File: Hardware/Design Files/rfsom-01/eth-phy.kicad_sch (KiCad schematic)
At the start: 45 parts, among them U6 KSZ9131RNXI-TR, Y1 ECS-2033-500-BN

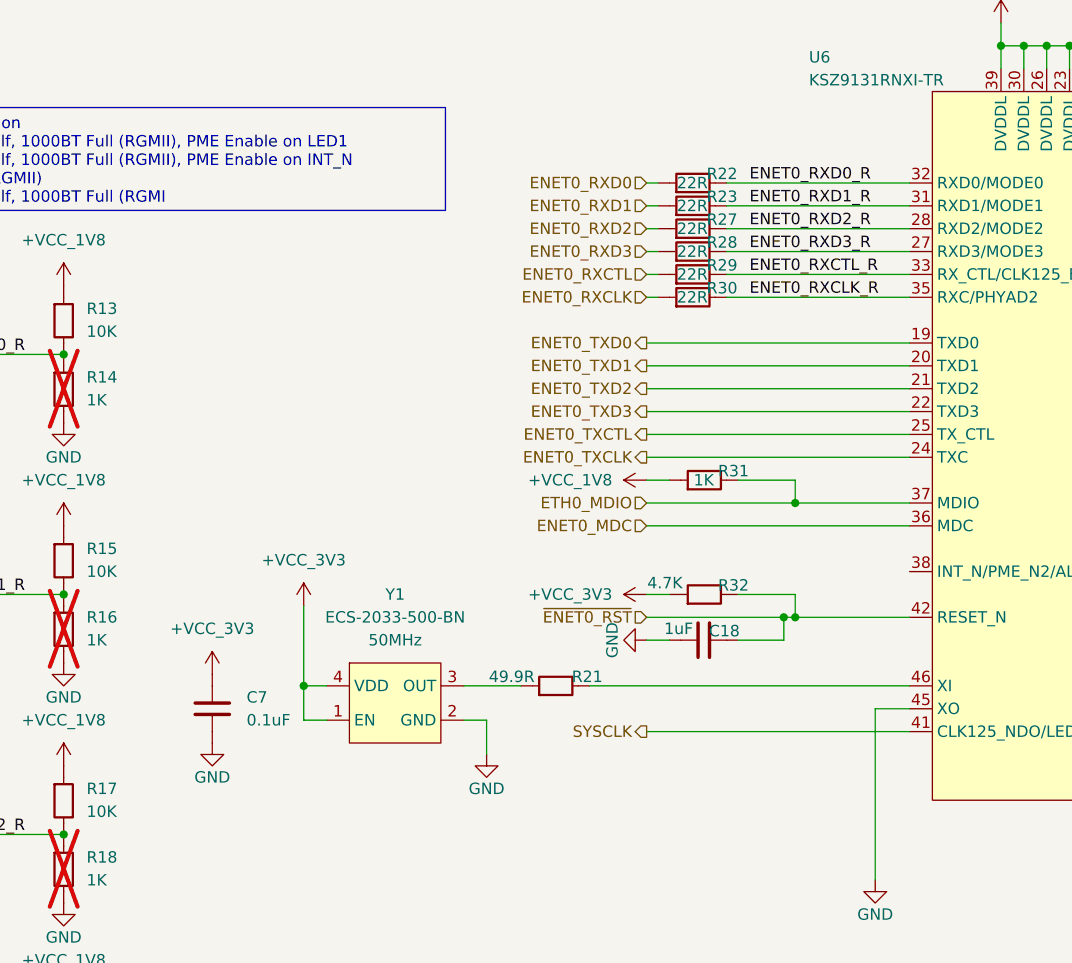
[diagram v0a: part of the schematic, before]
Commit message: added starage, usb sch; more design progress in sch;
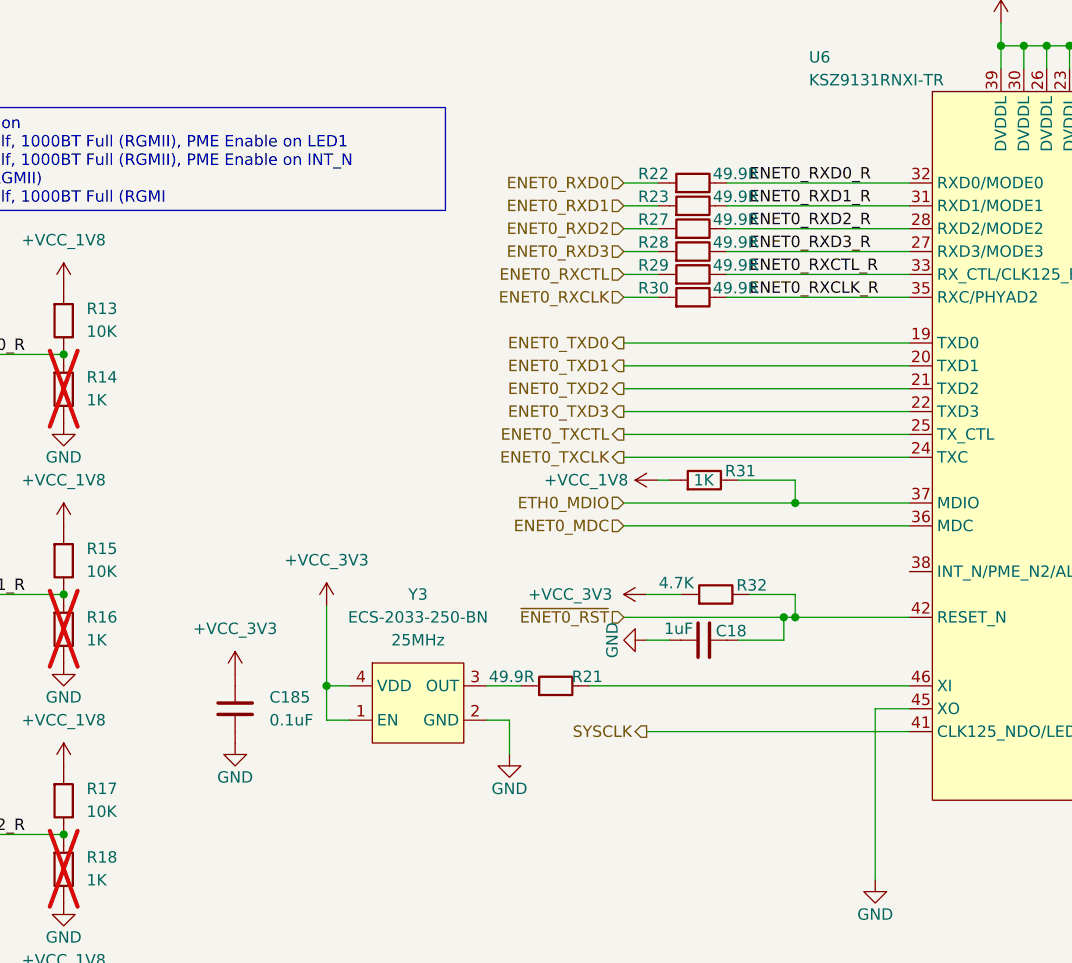
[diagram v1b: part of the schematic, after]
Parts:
- removed C7: CL05B104KA5NNNC, Capacitor_SMD:C_0402_1005Metric, symbol Capacitors:CL05B104KA5NNNC
- removed Y1: ECS-2033-500-BN, Miscellaneous:ECS-2033-500-BN, symbol Miscellaneous:ECS-2033-500-BN
- added C185: CL05B104KA5NNNC, Capacitor_SMD:C_0402_1005Metric, symbol Capacitors:CL05B104KA5NNNC
- added Y3: ECS-2033-250-BN, Miscellaneous:ECS-2033, symbol Miscellaneous:ECS-2033-250-BN
- R22, R23, R27, R28, R29, R30: footprint Resistor_SMD:R_0402_1005Metric -> Resistor_SMD:R_0603_1608Metric; symbol Resistors:RC0402FR-0722RL -> Resistors:RC0603FR-0749R9L; Resistance 22R -> 49.9R
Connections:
- net +VCC_3V3: now also C185.1, Y3.1 (EN), Y3.4 (VDD)
- net GND: now also C185.2, Y3.2 (GND)
- net at R21.1: now also Y3.3 (OUT)
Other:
- moved on the sheet: R32
